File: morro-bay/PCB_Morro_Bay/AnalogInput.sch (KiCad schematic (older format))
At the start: 117 parts, among them SW1 SW_DIP_x10, SW2 SW_DIP_x10, U10 LM2902, U11 LM2902, U12 LM2902, U5 LM2902, U6 LM2902, U7 LM2902, U8 LM2902, U9 LM2902

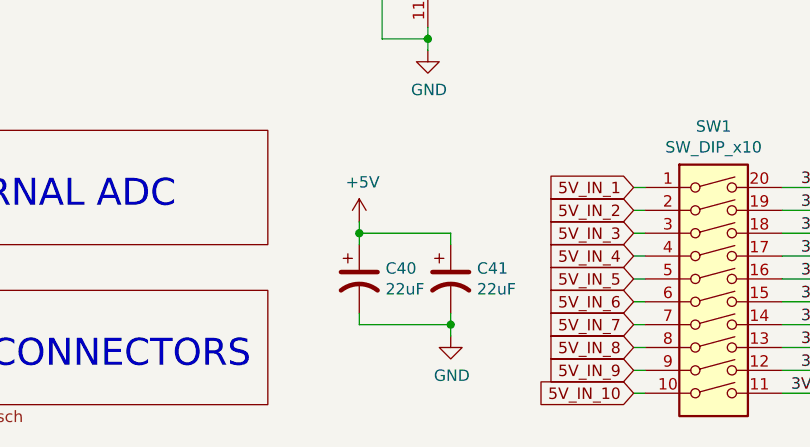
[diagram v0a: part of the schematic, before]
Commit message: More BOM
And if that don't work, use more gun.
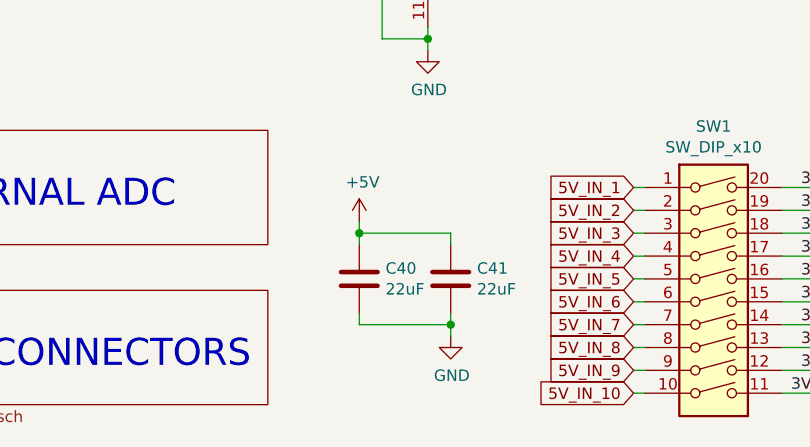
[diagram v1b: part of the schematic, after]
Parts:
- removed C40, C41: 22uF, symbol Device:CP1
- added C40, C41: 22uF, Capacitor_SMD:C_0805_2012Metric_Pad1.15x1.40mm_HandSolder, symbol Device:C
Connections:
- net +5V: now also C40.1, C41.1
- net GND: now also C40.2, C41.2
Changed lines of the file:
@@
-	1    0    0    -1
-$EndComp
-$Comp
-L Device:CP1 C40
-U 1 1 5EEAB869
-P 3050 7050
-F 0 "C40" H 3165 7096 50  0000 L CNN
-F 1 "22uF" H 3165 7005 50  0000 L CNN
-F 2 "" H 3050 7050 50  0001 C CNN
-F 3 "~" H 3050 7050 50  0001 C CNN
-	1    3050 7050
-	1    0    0    -1
-$EndComp
-$Comp
-L Device:CP1 C41
-U 1 1 5EEAD276
-P 3450 7050
-F 0 "C41" H 3565 7096 50  0000 L CNN
-F 1 "22uF" H 3565 7005 50  0000 L CNN
-F 2 "" H 3450 7050 50  0001 C CNN
-F 3 "~" H 3450 7050 50  0001 C CNN
-	1    3450 7050
 	1    0    0    -1
 $EndComp
@@
 	-1   0    0    1
 $EndComp
+$Comp
+L Device:C C?
+U 1 1 5E78EDE6
+P 3050 7050
+AR Path="/5E78EDE6" Ref="C?"  Part="1"
+AR Path="/5E59A680/5E78EDE6" Ref="C40"  Part="1"
+F 0 "C40" H 3165 7096 50  0000 L CNN
+F 1 "22uF" H 3165 7005 50  0000 L CNN
+F 2 "Capacitor_SMD:C_0805_2012Metric_Pad1.15x1.40mm_HandSolder" H 3088 6900 50  0001 C CNN
+F 3 "~" H 3050 7050 50  0001 C CNN
+F 4 "CL21A226MAQNNNE" H 3050 7050 50  0001 C CNN "Part Number"
+F 5 "https://www.digikey.ca/product-detail/en/samsung-electro-mechanics/CL21A226MAQNNNE/1276-2908-1-ND/3890994" H 3050 7050 50  0001 C CNN "Digikey"
+	1    3050 7050
+	1    0    0    -1
+$EndComp
+$Comp
+L Device:C C?
+U 1 1 5E7BDB3E
+P 3450 7050
+AR Path="/5E7BDB3E" Ref="C?"  Part="1"
+AR Path="/5E59A680/5E7BDB3E" Ref="C41"  Part="1"
+F 0 "C41" H 3565 7096 50  0000 L CNN
+F 1 "22uF" H 3565 7005 50  0000 L CNN
+F 2 "Capacitor_SMD:C_0805_2012Metric_Pad1.15x1.40mm_HandSolder" H 3488 6900 50  0001 C CNN
+F 3 "~" H 3450 7050 50  0001 C CNN
+F 4 "CL21A226MAQNNNE" H 3450 7050 50  0001 C CNN "Part Number"
+F 5 "https://www.digikey.ca/product-detail/en/samsung-electro-mechanics/CL21A226MAQNNNE/1276-2908-1-ND/3890994" H 3450 7050 50  0001 C CNN "Digikey"
+	1    3450 7050
+	1    0    0    -1
+$EndComp
 $EndSCHEMATC
